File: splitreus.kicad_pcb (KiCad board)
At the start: 2 copper layers, 127.5 x 99 mm, 68 parts, among them SW0 SW_PUSH, SW1 SW_PUSH, SW10 SW_PUSH, SW11 SW_PUSH, SW12 SW_PUSH, SW13 SW_PUSH, SW14 SW_PUSH, SW15 SW_PUSH, SW16 SW_PUSH, SW17 SW_PUSH, SW18 SW_PUSH, SW19 SW_PUSH, SW2 SW_PUSH, SW20 SW_PUSH, SW21 SW_PUSH, SW22 SW_PUSH, SW23 SW_PUSH, SW24 SW_PUSH, SW25 SW_PUSH, SW26 SW_PUSH, SW27 SW_PUSH, SW28 SW_PUSH, SW29 SW_PUSH, SW3 SW_PUSH, SW30 SW_PUSH, SW4 SW_PUSH, SW5 SW_PUSH, SW6 SW_PUSH, SW7 SW_PUSH, SW8 SW_PUSH, SW9 SW_PUSH, SW91 SW_PUSH, U1 nice_nano, U2 HOLE, U3 HOLE, U4 HOLE, U5 HOLE

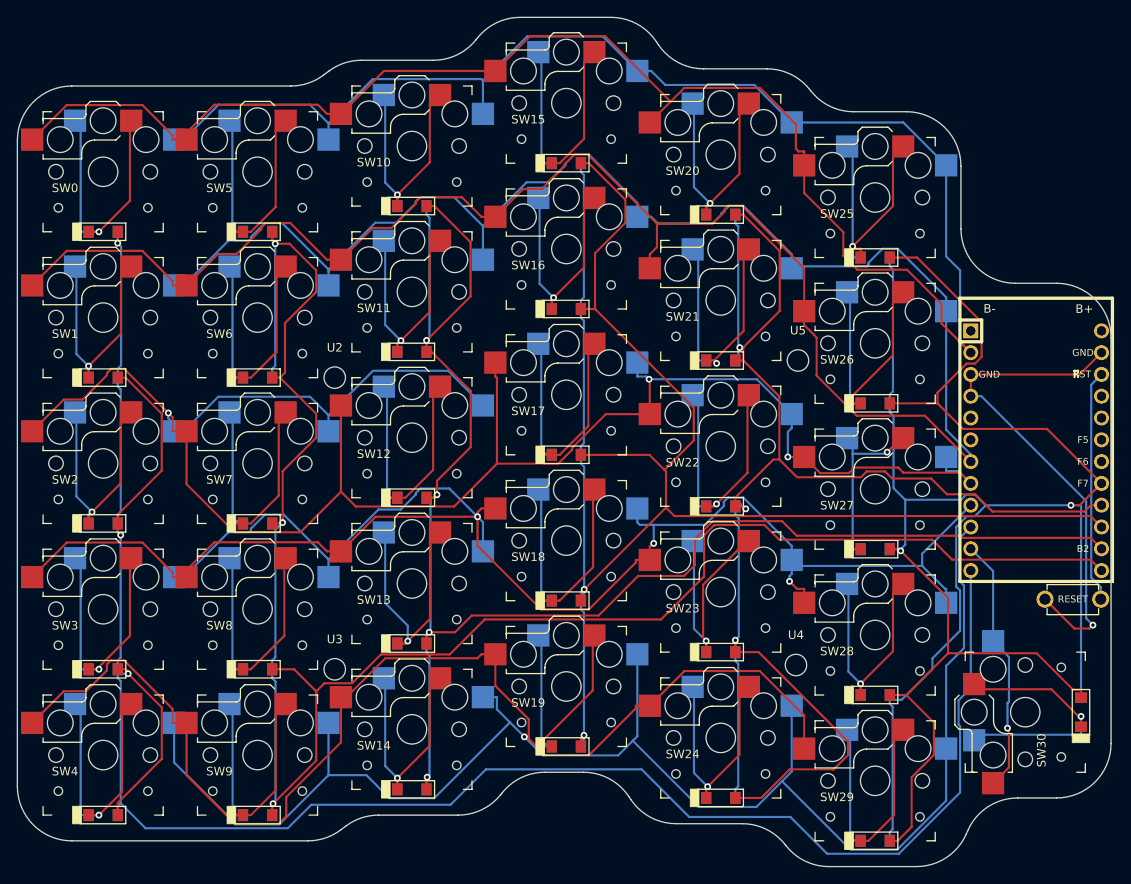
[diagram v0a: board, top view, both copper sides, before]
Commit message: upload
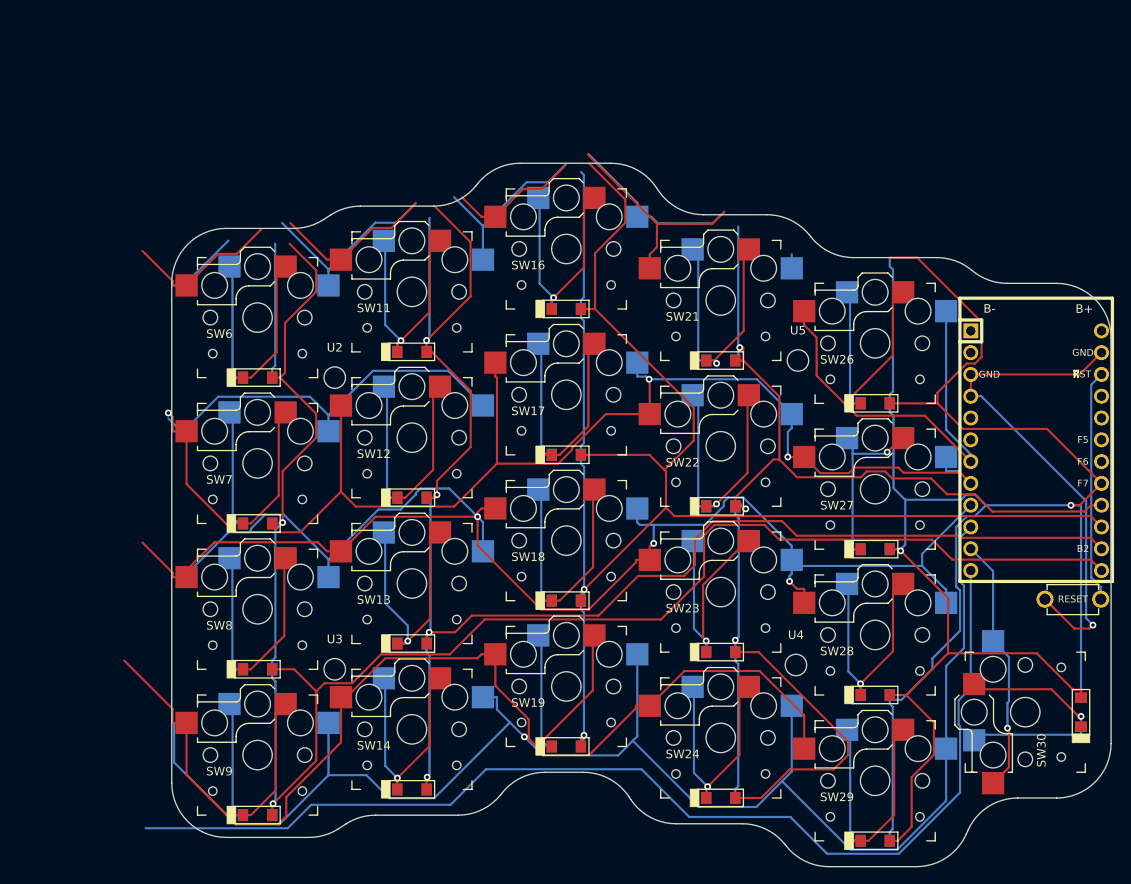
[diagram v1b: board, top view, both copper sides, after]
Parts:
- removed D0, D1, D10, D15, D2, D20, D25, D3, D4, D5: 1N4148-F, Custom Footies:smd_diode_reversible
- removed SW0, SW1, SW10, SW15, SW2, SW20, SW25, SW3, SW4, SW5: SW_PUSH, daprice_kail_mx:Kailh_socket_PG1350_reversible
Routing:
- net ROW0: track 279.5 -> 0.00 mm
- net COL0: track 252.3 -> 131.4 mm, vias 3 -> 0
- net ROW1: track 296.8 -> 202.2 mm
- net Net-(D5-Pad1): track 31.1 -> 0.00 mm, vias 1 -> 0
- net Net-(D3-Pad1): track 31.1 -> 0.00 mm, vias 1 -> 0
- net Net-(D4-Pad1): track 31.1 -> 0.00 mm, vias 1 -> 0
- net Net-(D0-Pad1): track 31.1 -> 0.00 mm, vias 1 -> 0
- net Net-(D15-Pad1): track 31.1 -> 0.00 mm, vias 1 -> 0
- net Net-(D25-Pad1): track 30.3 -> 0.00 mm, vias 1 -> 0
- net Net-(D20-Pad1): track 29.2 -> 0.00 mm, vias 1 -> 0
- net Net-(D2-Pad1): track 29.1 -> 0.00 mm, vias 1 -> 0
- net Net-(D10-Pad1): track 28.6 -> 0.00 mm, vias 1 -> 0
- net Net-(D1-Pad1): track 28.6 -> 0.00 mm, vias 1 -> 0
- net ROW2: track 223.0 -> 201.2 mm
- net COL4: track 175.7 -> 154.2 mm
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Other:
- board size 127.5 x 99 mm -> 109.5 x 82 mm
